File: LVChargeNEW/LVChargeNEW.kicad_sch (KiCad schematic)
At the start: 45 parts, among them Q1 CSD15380F3T, Q2 CSD15380F3T, Q3 CSD15380F3T, Q4 CSD15380F3T, U1 PQ25856QWRRVRQ1

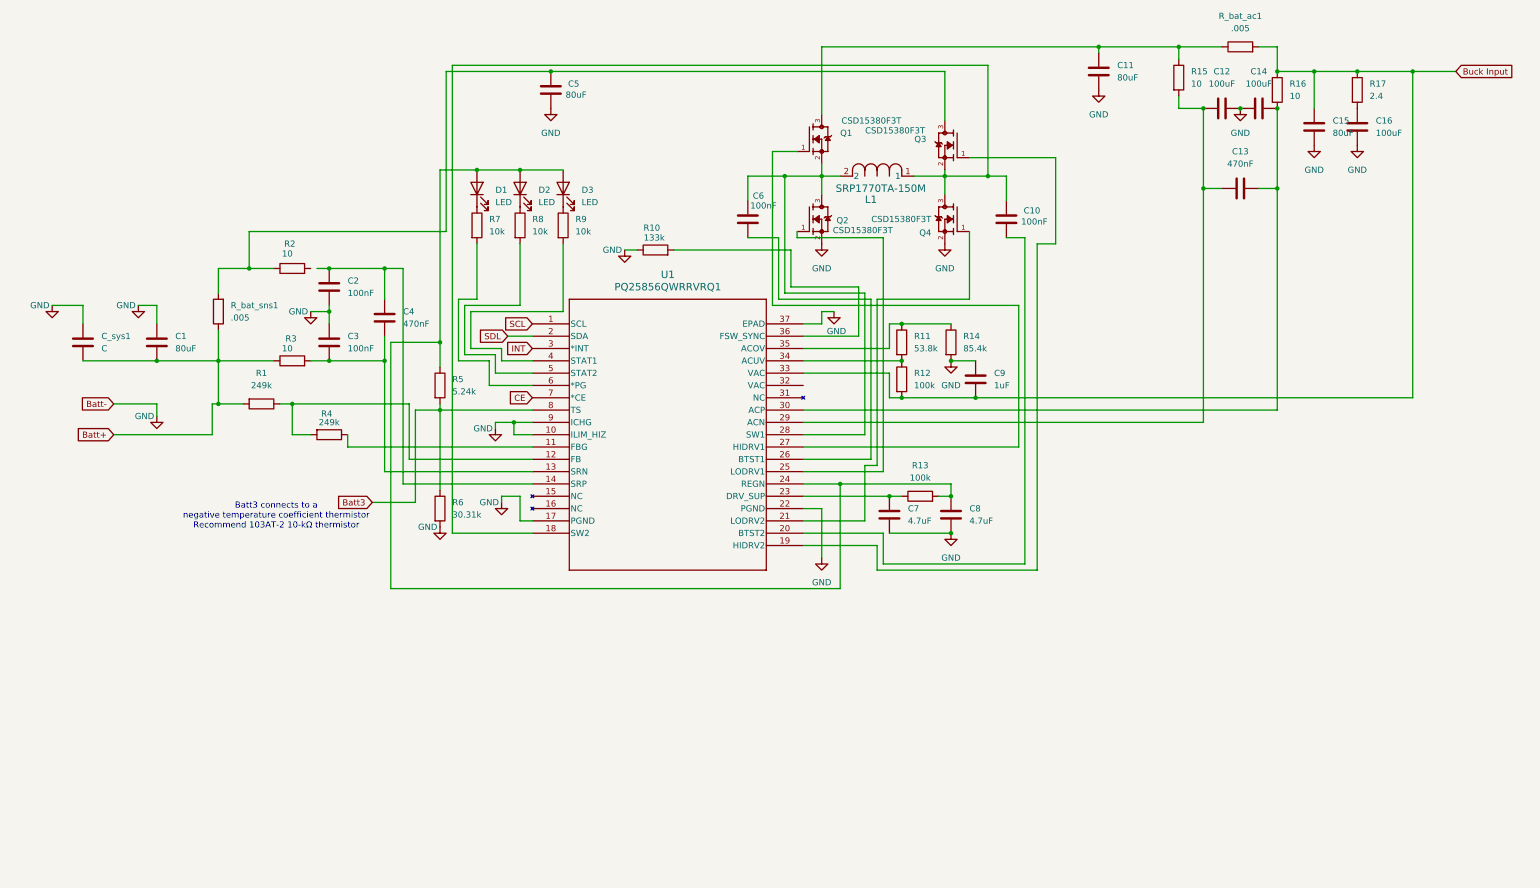
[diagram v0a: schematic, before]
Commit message: Updated GLVCharge Schematic
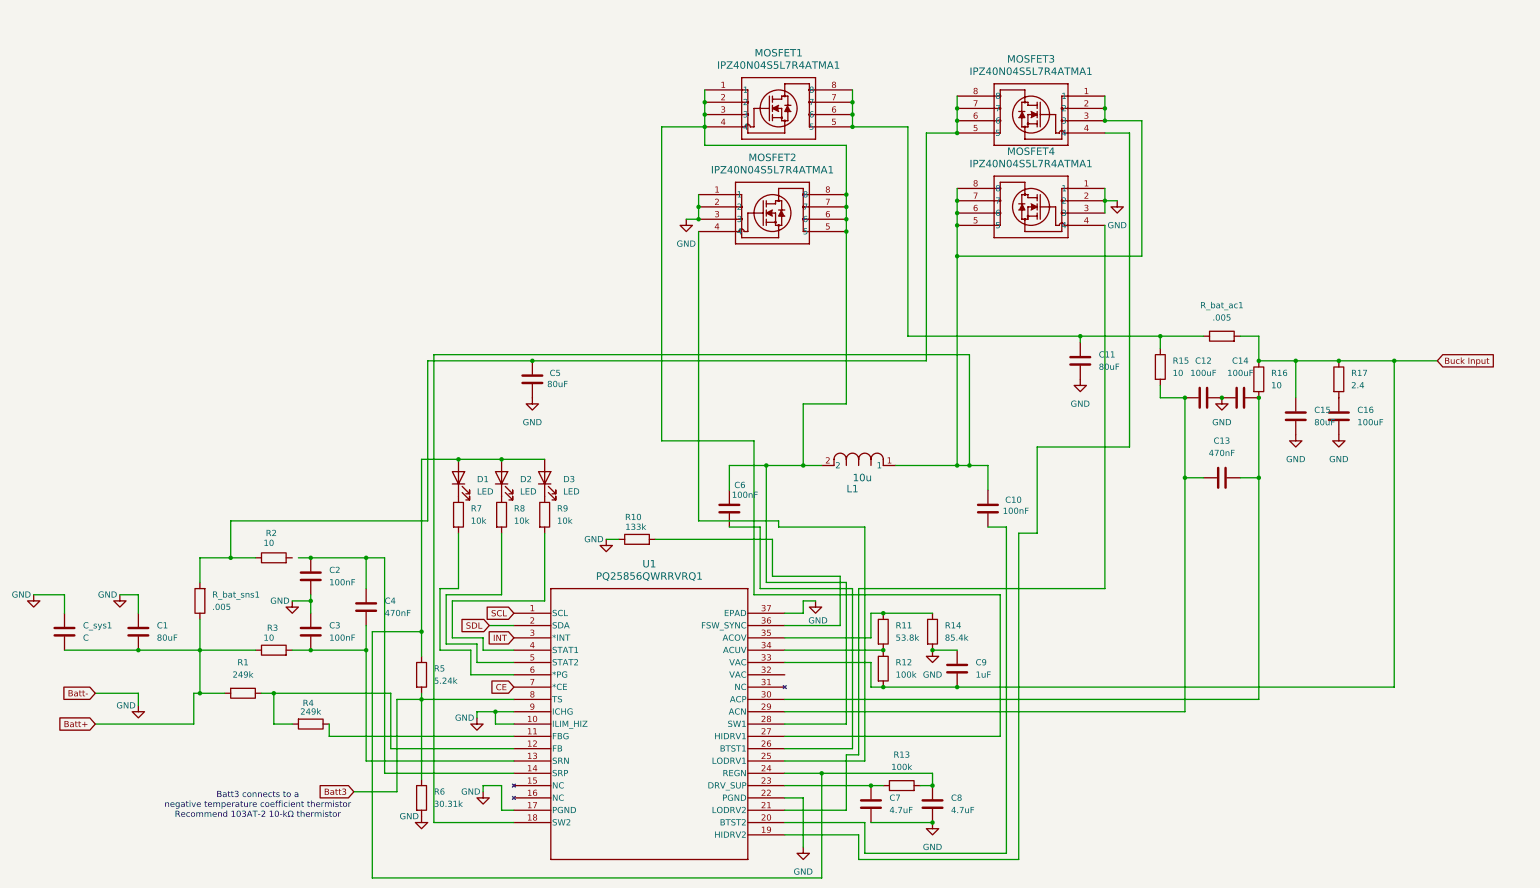
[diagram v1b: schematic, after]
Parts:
- removed Q1, Q2, Q3, Q4: CSD15380F3T, CSD15380F3T:TRXDFN69X60X35-3N, symbol LVChargeNEWLocalLib:CSD15380F3T
- added MOSFET1, MOSFET2, MOSFET3, MOSFET4: IPZ40N04S5L7R4ATMA1, mosfet:PG-TSDSON-8-32_INF, symbol 2025-10-30_20-54-56:IPZ40N04S5L7R4ATMA1
- L1: value SRP1770TA-150M -> 10u; footprint IND_SRP1770_BRN -> mosfet:inductor
- U1: footprint VQFN36_RRV_TEX -> chip:VQFN36_RRV_TEX
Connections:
- net GND: now also MOSFET2.1, MOSFET2.2, MOSFET2.3, MOSFET4.1, MOSFET4.2, MOSFET4.3
- net at U1.19 (HIDRV2): now also MOSFET3.4
- net at C10.2, L1.1, U1.18 (SW2): now also MOSFET3.1, MOSFET3.2, MOSFET3.3, MOSFET4.5, MOSFET4.6, MOSFET4.7, MOSFET4.8
- net at C5.2, R2.1, R_bat_sns1.2: now also MOSFET3.5, MOSFET3.6, MOSFET3.7, MOSFET3.8
- net at C6.2, L1.2, U1.28 (SW1): now also U1.27 (HIDRV1), MOSFET1.1, MOSFET1.2, MOSFET1.3, MOSFET1.4, MOSFET2.5, MOSFET2.6, MOSFET2.7, MOSFET2.8
- net at C11.2, R15.1, R_bat_ac1.1: now also MOSFET1.5, MOSFET1.6, MOSFET1.7, MOSFET1.8
- net at U1.25 (LODRV1): now also MOSFET2.4
- net at U1.21 (LODRV2): now also MOSFET4.4
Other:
- moved on the sheet: C1, C10, C11, C12, C13, C14, C15, C16, C2, C3, C4, C5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

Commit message: Uploaded Sean's stuff
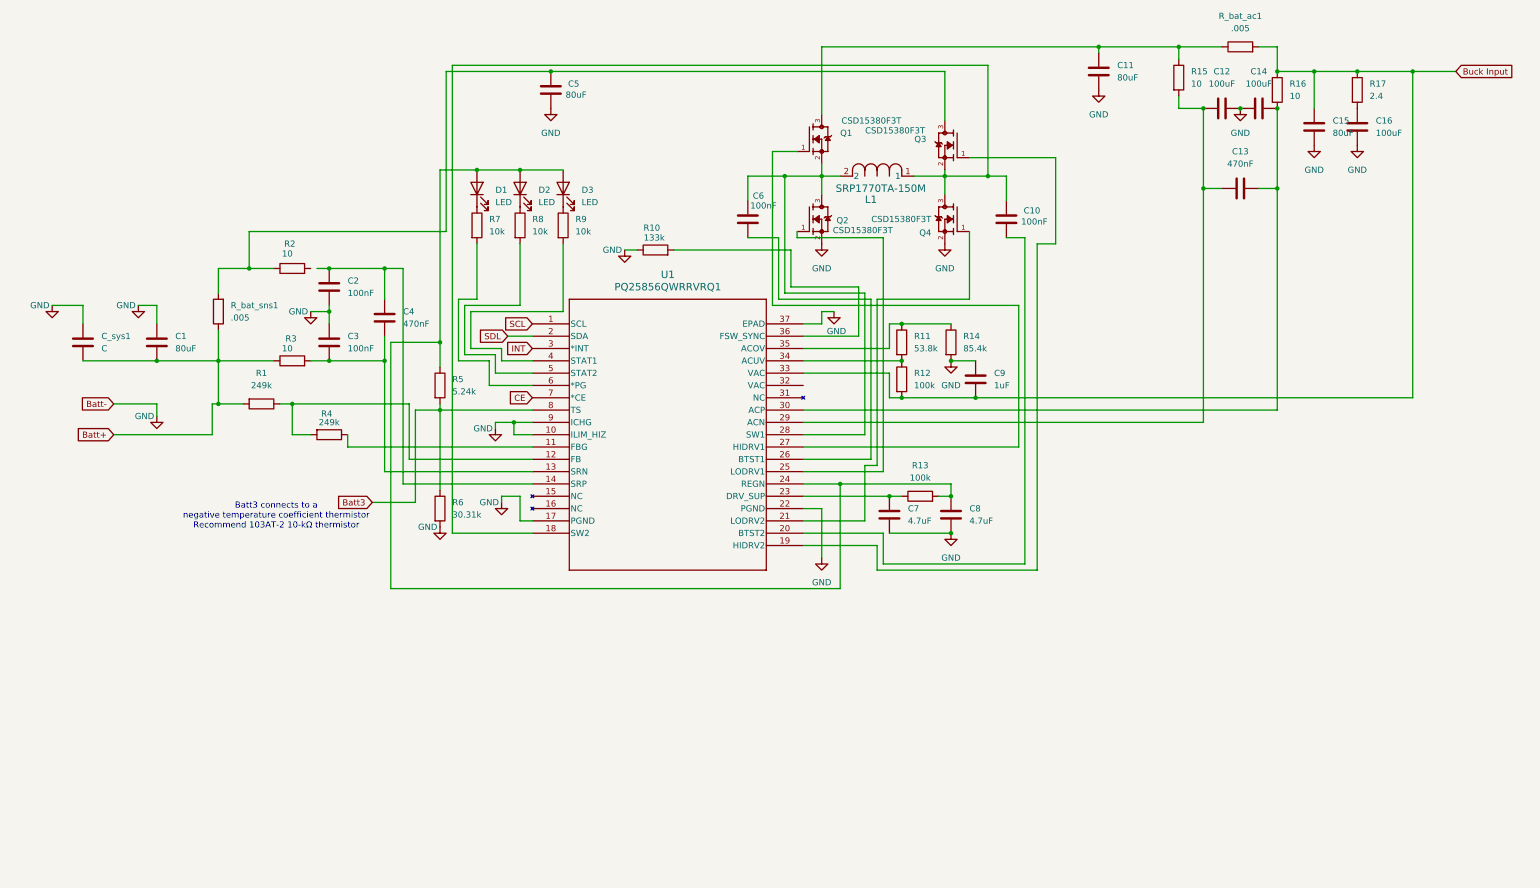
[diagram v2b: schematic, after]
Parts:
- removed MOSFET1, MOSFET2, MOSFET3, MOSFET4: IPZ40N04S5L7R4ATMA1, mosfet:PG-TSDSON-8-32_INF, symbol 2025-10-30_20-54-56:IPZ40N04S5L7R4ATMA1
- added Q1, Q2, Q3, Q4: CSD15380F3T, CSD15380F3T:TRXDFN69X60X35-3N, symbol LVChargeNEWLocalLib:CSD15380F3T
- L1: value 10u -> SRP1770TA-150M; footprint mosfet:inductor -> IND_SRP1770_BRN
- U1: footprint chip:VQFN36_RRV_TEX -> VQFN36_RRV_TEX
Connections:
- net GND: now also Q2.2, Q4.2
- net at U1.21 (LODRV2): now also Q4.1
- net at C10.2, L1.1, U1.18 (SW2): now also Q3.2, Q4.3
- net at C6.2, L1.2, U1.28 (SW1): now also Q1.2, Q2.3; no longer U1.27 (HIDRV1)
- net at C11.2, R15.1, R_bat_ac1.1: now also Q1.3
- net at U1.25 (LODRV1): now also Q2.1
- net at U1.19 (HIDRV2): now also Q3.1
- net at C5.2, R2.1, R_bat_sns1.2: now also Q3.3
- new net: Q1.1, U1.27 (HIDRV1)
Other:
- moved on the sheet: C1, C10, C11, C12, C13, C14, C15, C16, C2, C3, C4, C5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
